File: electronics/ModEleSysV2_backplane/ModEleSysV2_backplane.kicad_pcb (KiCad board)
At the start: 2 copper layers, 90 x 98 mm, 38 parts, among them J5 Conn_01x03, J6 Conn_01x03, J7 Conn_02x03_Odd_Even, J9 Conn_02x03_Odd_Even, SW1 switch_DPDT, SW2 switch_DPDT

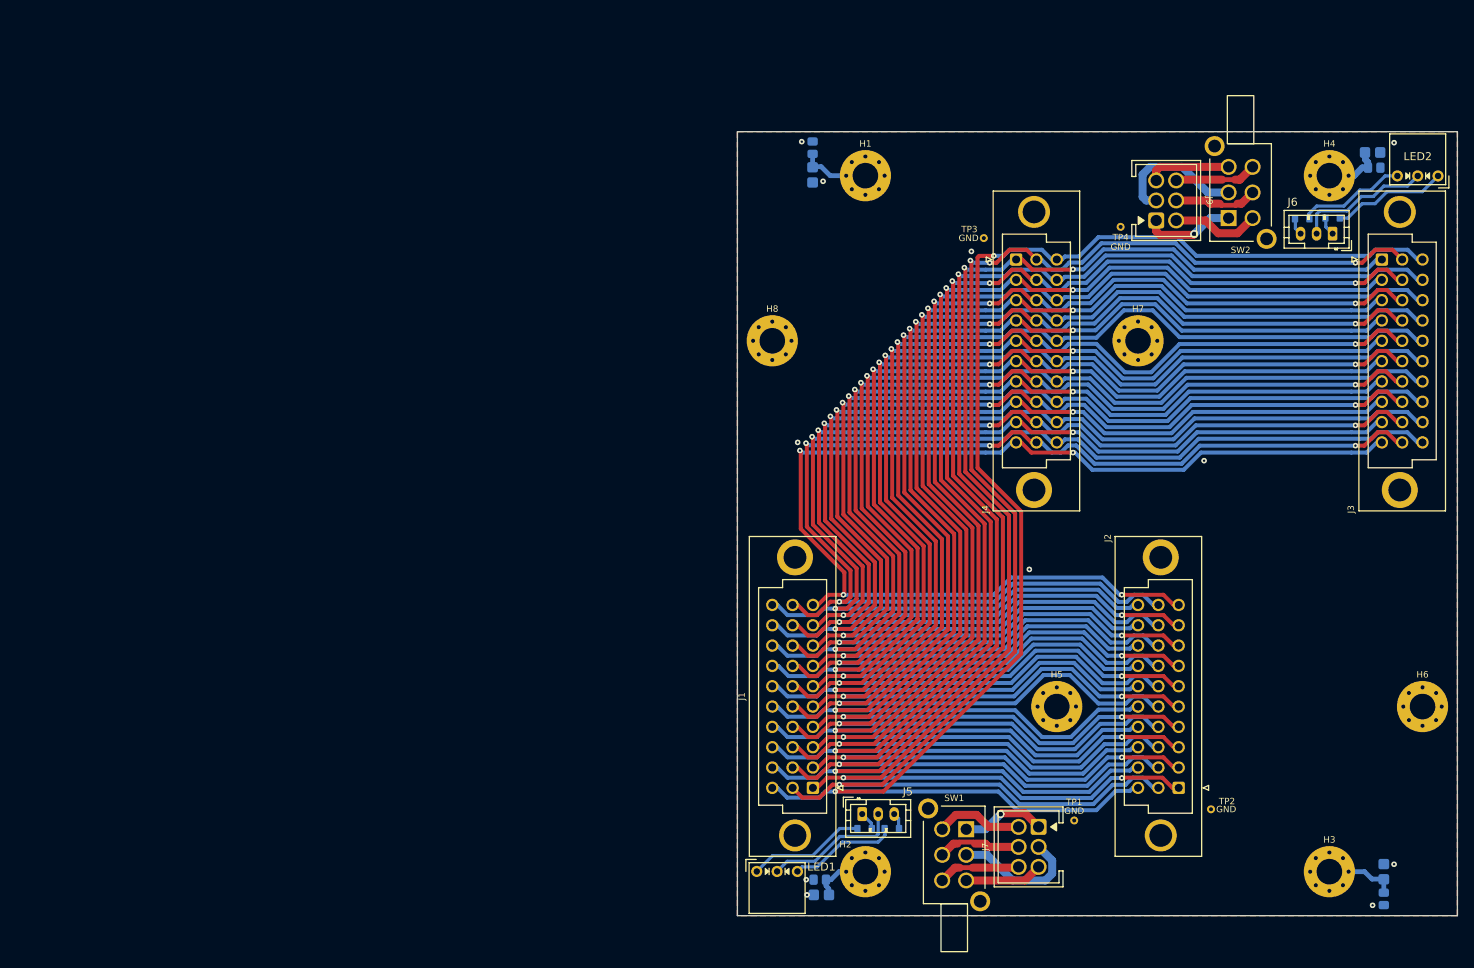
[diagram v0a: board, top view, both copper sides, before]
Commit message: reviewed and updated PCB's
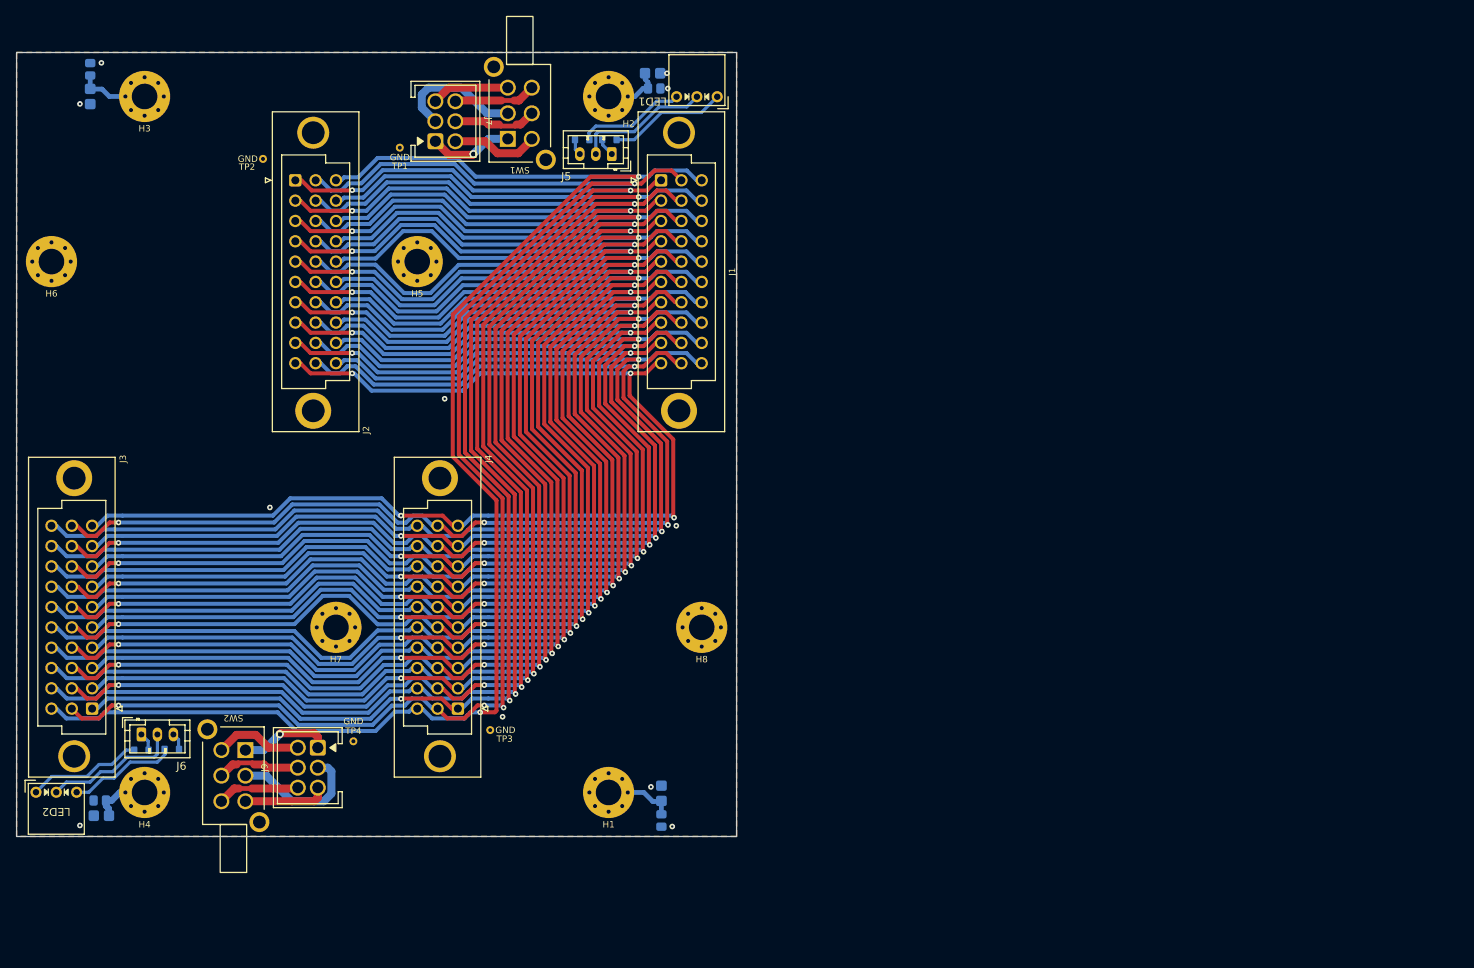
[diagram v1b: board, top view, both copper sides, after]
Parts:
- moved R3 192.1 mm to (39.2, 32.1), turned to 90 degrees
- moved C3 188.5 mm to (39.2, 35.5), turned to -90 degrees
- moved LED2 186.8 mm to (35.0, 122.5), turned to 0 degrees
- moved H6 180.2 mm to (34.4, 56.1), turned to 180 degrees
- moved C4 179.2 mm to (40.6, 125.4), turned to 180 degrees
- moved R4 177.9 mm to (40.4, 123.5), turned to 180 degrees
- moved H3 177.0 mm to (46.0, 35.5), turned to 180 degrees
- moved J3 169.6 mm to (36.9, 100.6), turned to 90 degrees
- moved H4 167.0 mm to (46.0, 122.5), turned to 180 degrees
- moved R7 163.1 mm to (45.6, 117.2), turned to 0 degrees
- moved J6 161.5 mm to (45.6, 115.2), turned to 0 degrees
- moved R8 156.1 mm to (49.4, 117.1), turned to 0 degrees
- moved SW2 145.5 mm to (57.1, 120.4), turned to -90 degrees
- moved TP2 143.7 mm to (60.8, 43.3), turned to 180 degrees
- moved J9 128.6 mm to (66.4, 119.4), turned to 90 degrees
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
